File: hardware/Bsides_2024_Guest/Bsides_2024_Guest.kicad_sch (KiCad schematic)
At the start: 44 parts, among them J1 Add_On, J2 Battery, J3 Battery, J4 OLED, J5 Conn_01x05, J6 Conn_01x05, P1 USB_C_Plug_USB2.0, Q1 DMG3415U-7, SW1 ON, SW2 RESET, SW3 BOOT, SW4 RESET, SW6 RESET, U1 ESP32-C6-WROOM-1U-N4, U2 AP2112K-3.3

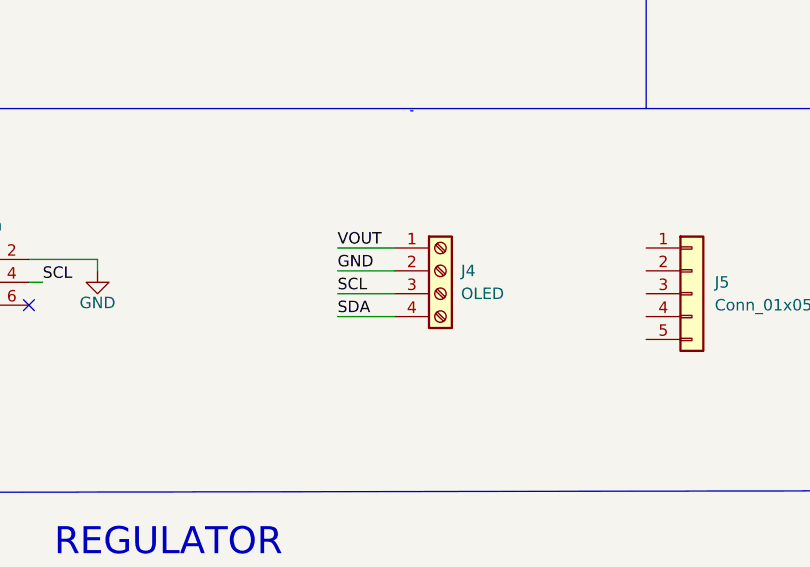
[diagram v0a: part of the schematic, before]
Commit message: feat(Hw): Update schematics
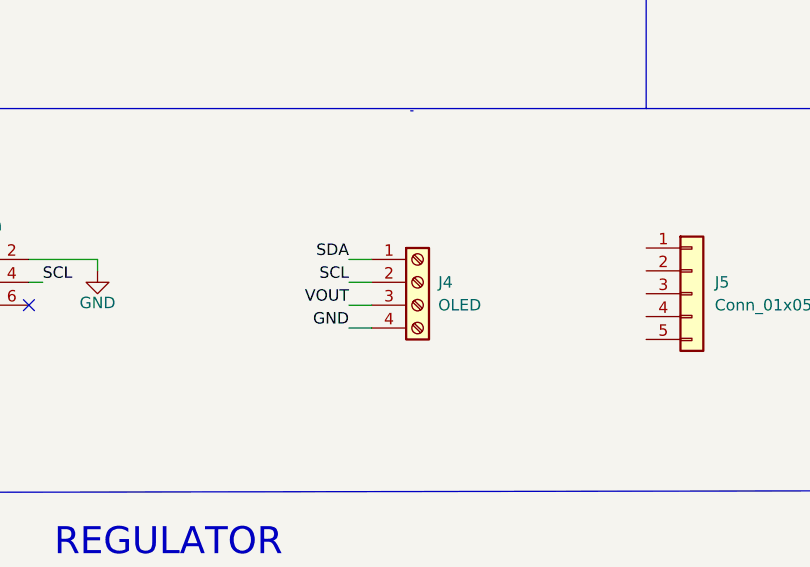
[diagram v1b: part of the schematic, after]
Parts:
- J4: manf# I2C SH1106 Display Oled Azul 128×64 1.3 ” -> Display OLED 128×32 0.91 I2C SSD1306 Blanco / Azul
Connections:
- net GND: now also J4.4 (Pin_4); no longer J4.2 (Pin_2)
- net SCL: now also J4.2 (Pin_2); no longer J4.3 (Pin_3)
- net SDA: now also J4.1 (Pin_1); no longer J4.4 (Pin_4)
- net VOUT: now also J4.3 (Pin_3); no longer J4.1 (Pin_1)
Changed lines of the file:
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@@
 	(wire
 		(pts
-			(xy 76.2 118.11) (xy 82.55 118.11)
-		)
-		(stroke
-			(width 0)
-			(type default)
-		)
-	)
-	(wire
-		(pts
 			(xy 192.024 119.761) (xy 196.215 119.761)
 		)
@@
 	(wire
 		(pts
-			(xy 76.2 120.65) (xy 82.55 120.65)
-		)
-		(stroke
-			(width 0)
-			(type default)
-		)
-	)
-	(wire
-		(pts
 			(xy 199.136 69.85) (xy 199.136 70.358)
 		)
@@
 	(wire
 		(pts
+			(xy 80.01 116.84) (xy 77.47 116.84)
+		)
+		(stroke
+			(width 0)
+			(type default)
+		)
+	)
+	(wire
+		(pts
 			(xy 58.674 79.756) (xy 62.484 79.756)
 		)
@@
 	(wire
 		(pts
-			(xy 76.2 123.19) (xy 82.55 123.19)
-		)
-		(stroke
-			(width 0)
-			(type default)
-		)
-	)
-	(wire
-		(pts
 			(xy 58.674 37.846) (xy 70.612 37.846)
 		)
@@
 	(wire
 		(pts
+			(xy 80.01 119.38) (xy 77.47 119.38)
+		)
+		(stroke
+			(width 0)
+			(type default)
+		)
+	)
+	(wire
+		(pts
 			(xy 262.89 119.761) (xy 266.7 119.761)
 		)
@@
 	(wire
 		(pts
-			(xy 76.2 115.57) (xy 82.55 115.57)
-		)
-		(stroke
-			(width 0)
-			(type default)
-		)
-	)
-	(wire
-		(pts
 			(xy 26.67 116.84) (xy 29.21 116.84)
 		)
@@
 	(wire
 		(pts
+			(xy 80.01 121.92) (xy 77.47 121.92)
+		)
+		(stroke
+			(width 0)
+			(type default)
+		)
+	)
+	(wire
+		(pts
 			(xy 251.587 89.154) (xy 251.587 85.598)
 		)
@@
 	(wire
 		(pts
+			(xy 80.01 124.46) (xy 77.47 124.46)
+		)
+		(stroke
+			(width 0)
+			(type default)
+		)
+	)
+	(wire
+		(pts
 			(xy 237.49 119.761) (xy 241.808 119.761)
 		)
@@
 		)
 	)
-	(label "SDA"
-		(at 76.2 123.19 0)
-		(fields_autoplaced yes)
-		(effects
-			(font
-				(size 1.27 1.27)
-			)
-			(justify left bottom)
-		)
-	)
 	(label "VOUT"
 		(at 213.36 118.11 0)
@@
 		)
 	)
-	(label "SCL"
-		(at 76.2 120.65 0)
-		(fields_autoplaced yes)
-		(effects
-			(font
-				(size 1.27 1.27)
-			)
-			(justify left bottom)
-		)
-	)
 	(label "PIN"
 		(at 172.466 131.826 0)
@@
 		)
 	)
-	(label "GND"
-		(at 76.2 118.11 0)
+	(label "D+"
+		(at 149.606 59.69 0)
 		(fields_autoplaced yes)
 		(effects
@@
 		)
 	)
-	(label "D+"
-		(at 149.606 59.69 0)
+	(label "D-"
+		(at 29.972 65.786 0)
 		(fields_autoplaced yes)
 		(effects
@@
 		)
 	)
-	(label "D-"
-		(at 29.972 65.786 0)
+	(label "SCL"
+		(at 77.47 119.38 180)
 		(fields_autoplaced yes)
 		(effects
@@
 				(size 1.27 1.27)
 			)
-			(justify left bottom)
+			(justify right bottom)
 		)
 	)
@@
 		)
 	)
+	(label "GND"
+		(at 77.47 124.46 180)
+		(fields_autoplaced yes)
+		(effects
+			(font
+				(size 1.27 1.27)
+			)
+			(justify right bottom)
+		)
+	)
 	(label "BOOT"
 		(at 182.753 67.818 180)
@@
 		)
 	)
-	(label "VOUT"
-		(at 76.2 115.57 0)
-		(fields_autoplaced yes)
-		(effects
-			(font
-				(size 1.27 1.27)
-			)
-			(justify left bottom)
-		)
-	)
 	(label "GPIO15"
 		(at 62.484 71.374 0)
@@
 		)
 	)
+	(label "SDA"
+		(at 77.47 116.84 180)
+		(fields_autoplaced yes)
+		(effects
+			(font
+				(size 1.27 1.27)
+			)
+			(justify right bottom)
+		)
+	)
 	(label "VOUT"
 		(at 85.09 58.42 0)
@@
 		)
 	)
+	(label "VOUT"
+		(at 77.47 121.92 180)
+		(fields_autoplaced yes)
+		(effects
+			(font
+				(size 1.27 1.27)
+			)
+			(justify right bottom)
+		)
+	)
 	(label "BOOT"
 		(at 24.638 71.374 0)
@@
 	)
 	(symbol
+		(lib_id "Connector:Screw_Terminal_01x04")
+		(at 85.09 119.38 0)
+		(unit 1)
+		(exclude_from_sim no)
+		(in_bom yes)
+		(on_board yes)
+		(dnp no)
+		(fields_autoplaced yes)
+		(property "Reference" "J4"
+			(at 87.376 119.3799 0)
+			(effects
+				(font
+					(size 1.27 1.27)
+				)
+				(justify left)
+			)
+		)
+		(property "Value" "OLED"
+			(at 87.376 121.9199 0)
+			(effects
+				(font
+					(size 1.27 1.27)
+				)
+				(justify left)
+			)
+		)
+		(property "Footprint" "bsides:Display OLED 128 x32"
+			(at 85.09 119.38 0)
+			(effects
+				(font
+					(size 1.27 1.27)
+				)
+				(hide yes)
+			)
+		)
+		(property "Datasheet" ""
+			(at 85.09 119.38 0)
+			(effects
+				(font
+					(size 1.27 1.27)
+				)
+				(hide yes)
+			)
+		)
+		(property "Description" ""
+			(at 85.09 119.38 0)
+			(effects
+				(font
+					(size 1.27 1.27)
+				)
+				(hide yes)
+			)
+		)
+		(property "manf#" "Display OLED 128×32 0.91 I2C SSD1306 Blanco / Azul"
+			(at 85.09 119.38 0)
+			(effects
+				(font
+					(size 1.27 1.27)
+				)
+				(hide yes)
+			)
+		)
+		(property "provedor" "UNIT Electronics"
+			(at 85.09 119.38 0)
+			(effects
+				(font
+					(size 1.27 1.27)
+				)
+				(hide yes)
+			)
+		)
+		(pin "1"
+		)
+		(pin "2"
+		)
+		(pin "3"
+		)
+		(pin "4"
+		)
+		(instances
+			(project "Bsides_2024_Guest"
+				(path "/21a57a81-777f-4f81-b806-a7171bf6ef6c"
+					(reference "J4")
+					(unit 1)
+				)
+			)
+		)
+	)
+	(symbol
 		(lib_id "power:GND")
 		(at 199.39 55.88 0)
@@
 					(unit 1)
 				)
-			)
-		)
-	)
-	(symbol
-		(lib_id "Connector:Screw_Terminal_01x04")
-		(at 87.63 118.11 0)
-		(unit 1)
-		(exclude_from_sim no)
-		(in_bom yes)
-		(on_board yes)
-		(dnp no)
-		(fields_autoplaced yes)
-		(property "Reference" "J4"
-			(at 89.916 118.1099 0)
-			(effects
-				(font
-					(size 1.27 1.27)
-				)
-				(justify left)
-			)
-		)
-		(property "Value" "OLED"
-			(at 89.916 120.6499 0)
-			(effects
-				(font
-					(size 1.27 1.27)
-				)
-				(justify left)
-			)
-		)
-		(property "Footprint" "bsides:Display OLED 128 x32"
-			(at 87.63 118.11 0)
-			(effects
-				(font
-					(size 1.27 1.27)
-				)
-				(hide yes)
-			)
-		)
-		(property "Datasheet" "~"
-			(at 87.63 118.11 0)
-			(effects
-				(font
-					(size 1.27 1.27)
-				)
-				(hide yes)
-			)
-		)
-		(property "Description" ""
-			(at 87.63 118.11 0)
-			(effects
-				(font
-					(size 1.27 1.27)
-				)
-				(hide yes)
-			)
-		)
-		(property "manf#" "I2C SH1106 Display Oled Azul 128×64 1.3 ” "
-			(at 87.63 118.11 0)
-			(effects
-				(font
-					(size 1.27 1.27)
-				)
-				(hide yes)
-			)
-		)
-		(property "provedor" "UNIT Electronics"
-			(at 87.63 118.11 0)
-			(effects
-				(font
-					(size 1.27 1.27)
-				)
-				(hide yes)
-			)
-		)
-		(pin "1"
-		)
-		(pin "2"
-		)
-		(pin "3"
-		)
-		(pin "4"
-		)
-		(instances
-			(project "Bsides_2024_Guest"
-				(path "/21a57a81-777f-4f81-b806-a7171bf6ef6c"
-					(reference "J4")
-					(unit 1)
-				)
